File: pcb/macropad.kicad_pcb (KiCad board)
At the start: 2 copper layers, 70 x 64.5 mm, 15 parts, among them SW1 SW_Push, SW2 SW_Push, SW3 SW_Push, SW4 SW_Push, SW5 SW_Push, SW6 SW_Push, U1 SEEED STUDIO XIAO RP2040, U2 1x0.91 IN. OLED

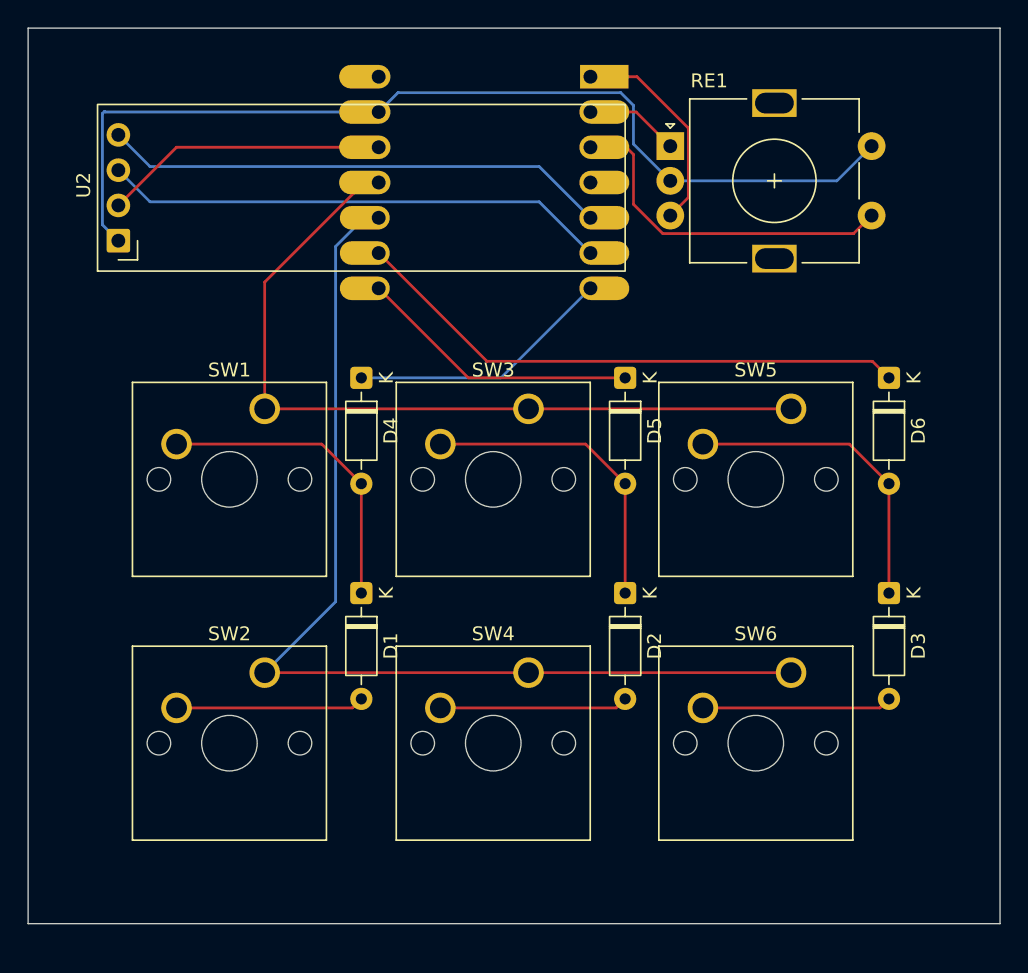
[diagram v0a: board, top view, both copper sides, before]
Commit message: Update images without display
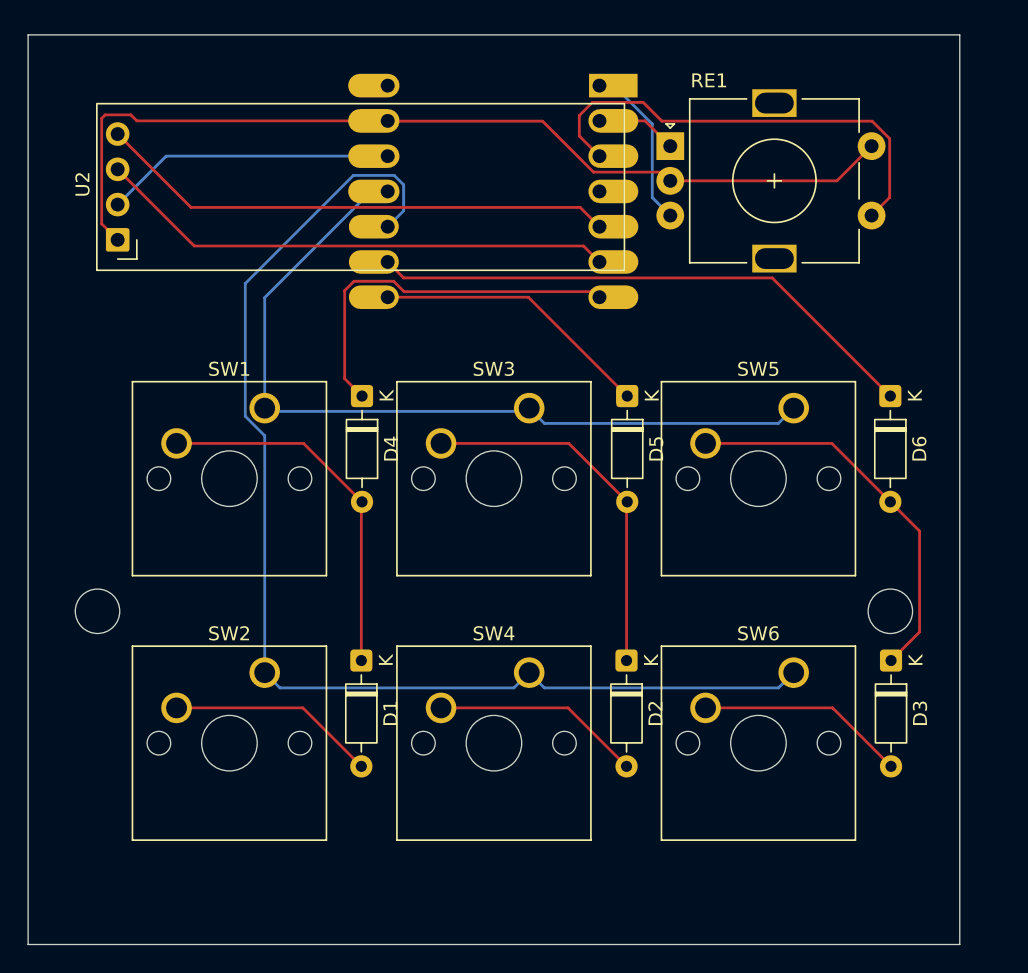
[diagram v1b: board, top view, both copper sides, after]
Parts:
- added REF**: MountingHole_3.2mm_M3, MountingHole:MountingHole_3.2mm_M3, F.Cu at (100.0, 69.0)
- added REF**: MountingHole_3.2mm_M3, MountingHole:MountingHole_3.2mm_M3, F.Cu at (157.1, 69.0)
- moved D3 4.86 mm to (157.2, 72.5)
- moved D2 4.86 mm to (138.1, 72.5)
- moved D1 4.86 mm to (119.0, 72.5)
- moved D5 1.32 mm to (138.2, 53.5)
- moved D6 1.31 mm to (157.1, 53.5)
- moved D4 1.31 mm to (119.0, 53.5)
- moved U1 0.91 mm to (128.5, 38.8)
- moved SW5 0.20 mm to (150.1, 54.4)
- moved SW6 0.19 mm to (150.1, 73.4)
- moved U2 0.08 mm to (101.5, 42.2)
- moved SW3 0.07 mm to (131.1, 54.4)
- moved SW4 0.05 mm to (131.1, 73.4)
- moved SW1 0.05 mm to (112.0, 54.4)
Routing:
- net Net-(U1-PA5_A9_D9_MISO): track 73.6 -> 86.9 mm
- net Net-(U1-PA10_A2_D2): track 22.9 -> 33.4 mm
- net Net-(D4-K): track 19.2 -> 27.2 mm
- net Net-(D3-K): track 22.5 -> 28.2 mm
- net Net-(D2-K): track 22.4 -> 26.6 mm
- net Net-(D1-K): track 22.4 -> 26.6 mm
- net Net-(U1-PA02_A0_D0): track 15.4 -> 12.1 mm
- net GND: track 71.0 -> 67.8 mm
- net Net-(U1-PA6_A10_D10_MOSI): track 57.2 -> 59.2 mm
- net Net-(D2-A): track 13.6 -> 15.1 mm
- net Net-(D1-A): track 13.6 -> 15.1 mm
- net Net-(D3-A): track 13.7 -> 15.1 mm
- net Net-(U1-PA9_A5_D5_SCL): track 36.5 -> 37.5 mm
- net Net-(U1-PA8_A4_D4_SDA): track 36.5 -> 37.5 mm
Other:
- board size 70 x 64.5 mm -> 67.1 x 65.5 mm
